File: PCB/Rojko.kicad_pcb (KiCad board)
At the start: 2 copper layers, 20 x 20 mm, 36 parts, among them IC3 AP63203WU-7, IC4 STM32WB35CEU6A, J1 AYF-531035, J6 AYF-531035, SW3 SW_MEC_5G, Y2 Crystal_GND24, Y3 32,768k

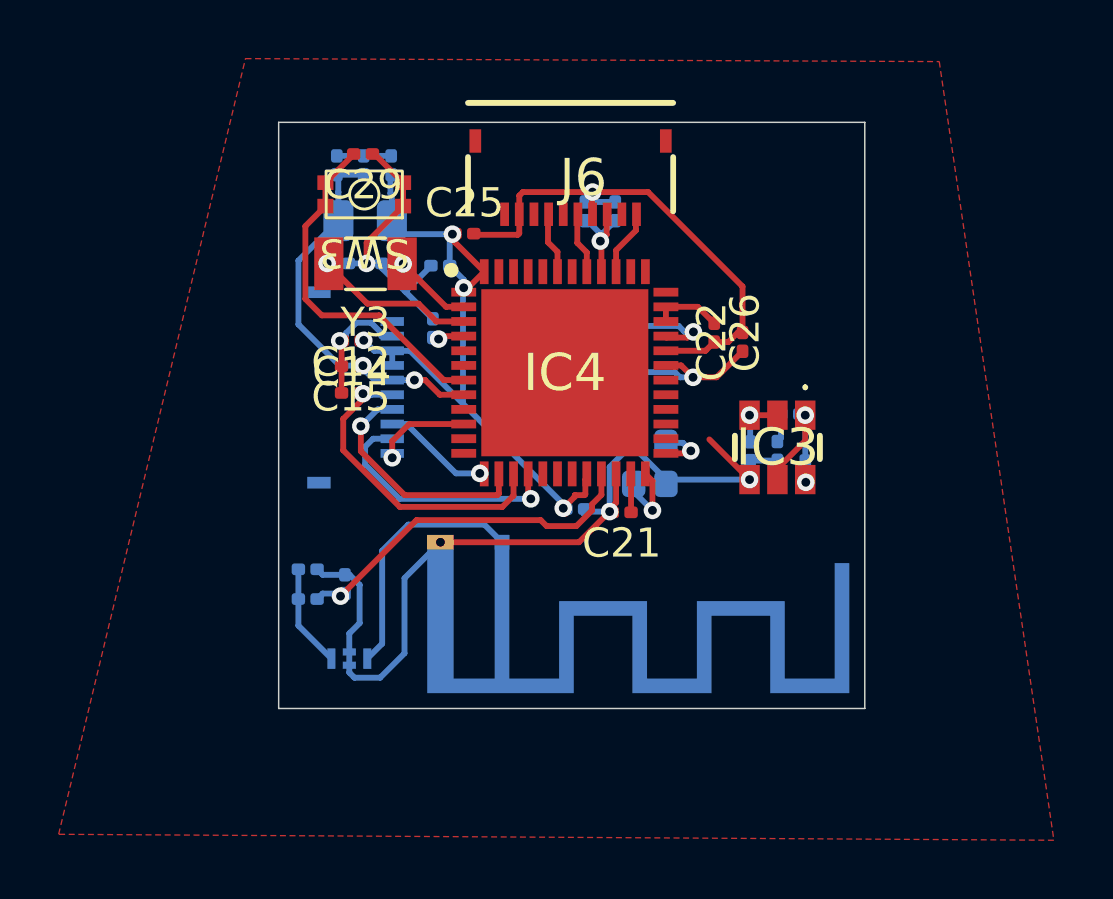
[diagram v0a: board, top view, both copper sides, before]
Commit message: dwa
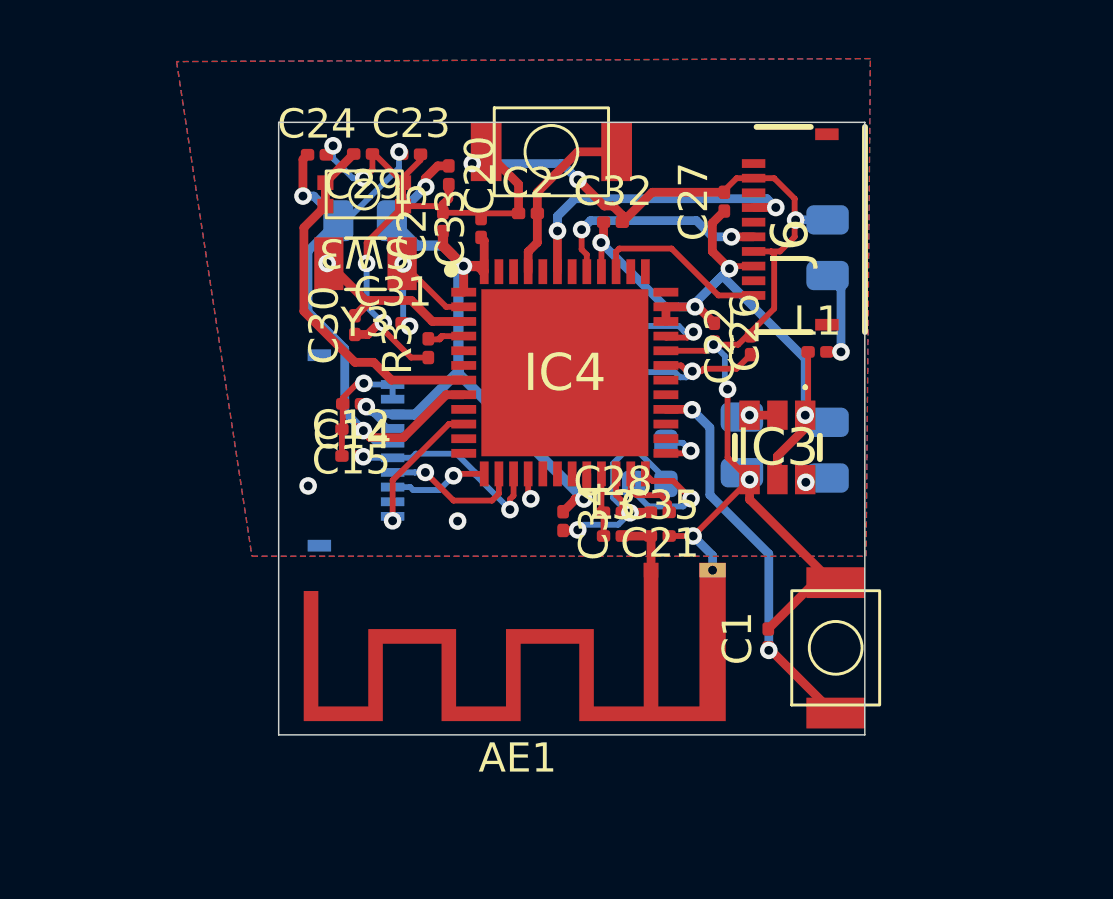
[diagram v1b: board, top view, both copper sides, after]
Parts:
- removed FL1: DLF162500LT-5028A1, DLF162500LT-5028A1:DLF162500LT5028A1
- added C1: 100nF, Capacitor_SMD:C_0201_0603Metric, F.Cu at (113.8, 100.4)
- added C2: 100nF, Capacitor_SMD:C_0201_0603Metric, F.Cu at (105.6, 85.9)
- added SW1: SW_MEC_5G, CUSTOM:Switch small but not that small, F.Cu at (116.1, 100.7)
- added SW2: SW_MEC_5G, CUSTOM:Switch small but not that small, F.Cu at (106.4, 83.8)
- AE1, C20, C23, C24, C27, C28, C30, C31, C32, C33, C34, C35, L1, L3, R3: moved to F.Cu
- C16, C17, C18: footprint Capacitor_SMD:C_0201_0603Metric -> Capacitor_SMD:C_0805_2012Metric
- moved C35 12.1 mm to (110.1, 96.9)
- moved L3 10.6 mm to (108.5, 96.9), turned to 0 degrees
- moved C28 9.47 mm to (108.5, 96.1), turned to 0 degrees
- moved C17 7.14 mm to (115.8, 87.1), turned to -90 degrees
- moved J6 6.38 mm to (113.4, 86.5), turned to 90 degrees
- moved AE1 5.17 mm to (109.8, 98.1), turned to 180 degrees
- moved C27 3.74 mm to (112.3, 85.5)
- moved L1 2.31 mm to (115.5, 90.6), turned to 0 degrees
- moved C30 2.17 mm to (99.7, 89.7), turned to 90 degrees
- moved C14 2.15 mm to (99.6, 92.4)
- moved C12 2.15 mm to (99.6, 94.2)
- moved C15 2.15 mm to (99.6, 93.3)
- moved J1 2.15 mm to (100.9, 94.0)
- moved C31 2.03 mm to (101.0, 89.6)
- moved C20 2.00 mm to (102.9, 84.6), turned to -90 degrees
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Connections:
- AE1 pad 1: Net-(AE1-A) -> /RF
- C35 pad 1: Net-(FL1-IN) -> /RF
- IC4 pad 28: unconnected-(IC4-PB0-Pad28) -> Net-(IC4-PB0)
- IC4 pad 29: BAT_GPO -> unconnected-(IC4-PB1-Pad29)
- IC4 pad 45: unconnected-(IC4-PB5-Pad45) -> Net-(IC4-PB5)
- L3 pad 2: Net-(FL1-IN) -> /RF
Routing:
- net +3.3V: track 34.5 -> 52.9 mm, vias 6 -> 8
- net Net-(IC4-PB0): track 0.00 -> 13.4 mm, vias 0 -> 2
- net GND: track 61.3 -> 73.1 mm, vias 4 -> 15
- net Net-(IC4-RF1): track 12.6 -> 2.19 mm, vias 1 -> 0
- net Net-(AE1-A): track 8.60 -> 0.00 mm
- net PROG_SWO: track 2.10 -> 10.6 mm, vias 0 -> 2
- net DISP_MOSI: track 8.71 -> 0.92 mm
- net +3.3VA: track 13.3 -> 20.4 mm, vias 2 -> 3
- net Net-(IC4-PB5): track 0.00 -> 6.11 mm
- net PROG_SWCLK: track 2.10 -> 7.73 mm, vias 0 -> 2
- net PROG_SWDIO: track 2.25 -> 6.08 mm
- net DISP_ON/OFF: track 10.7 -> 7.18 mm, vias 1 -> 2
- net Net-(FL1-IN): track 3.51 -> 0.00 mm
- net DISP_VCOM: track 8.19 -> 4.80 mm
- net Net-(C17-Pad2): track 0.99 -> 3.28 mm, vias 0 -> 1
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- added copper zone on B.Cu, net GND
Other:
- board size 20 x 20 mm -> 20 x 20.9 mm
